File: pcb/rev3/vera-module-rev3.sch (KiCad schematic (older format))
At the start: 120 parts, among them J1 Bus, J2 Prog, J3 SD_Card, J4 Composite, J5 VGA, J6 Conn_01x04, J7 Conn_01x02, J8 RS232, J9 S-video, U1 ICE40UP5K-SG48ITR50, U10 MIC5504-3.3YM5, U11 THS7314D, U12 MAX3221CPWR, U2 74AHC00PW, U3 SN74CBTD3861PWR, U4 74AHC1G14GW,125, U5 74LVC4245APW, U6 WM8524CGEDT, U7 W25Q16JVSNIQ, U8 74AHC1G14GW,125, U9 AP3417CKTR-G1, X1 SG5032CAN_25.000000M-TJGA3

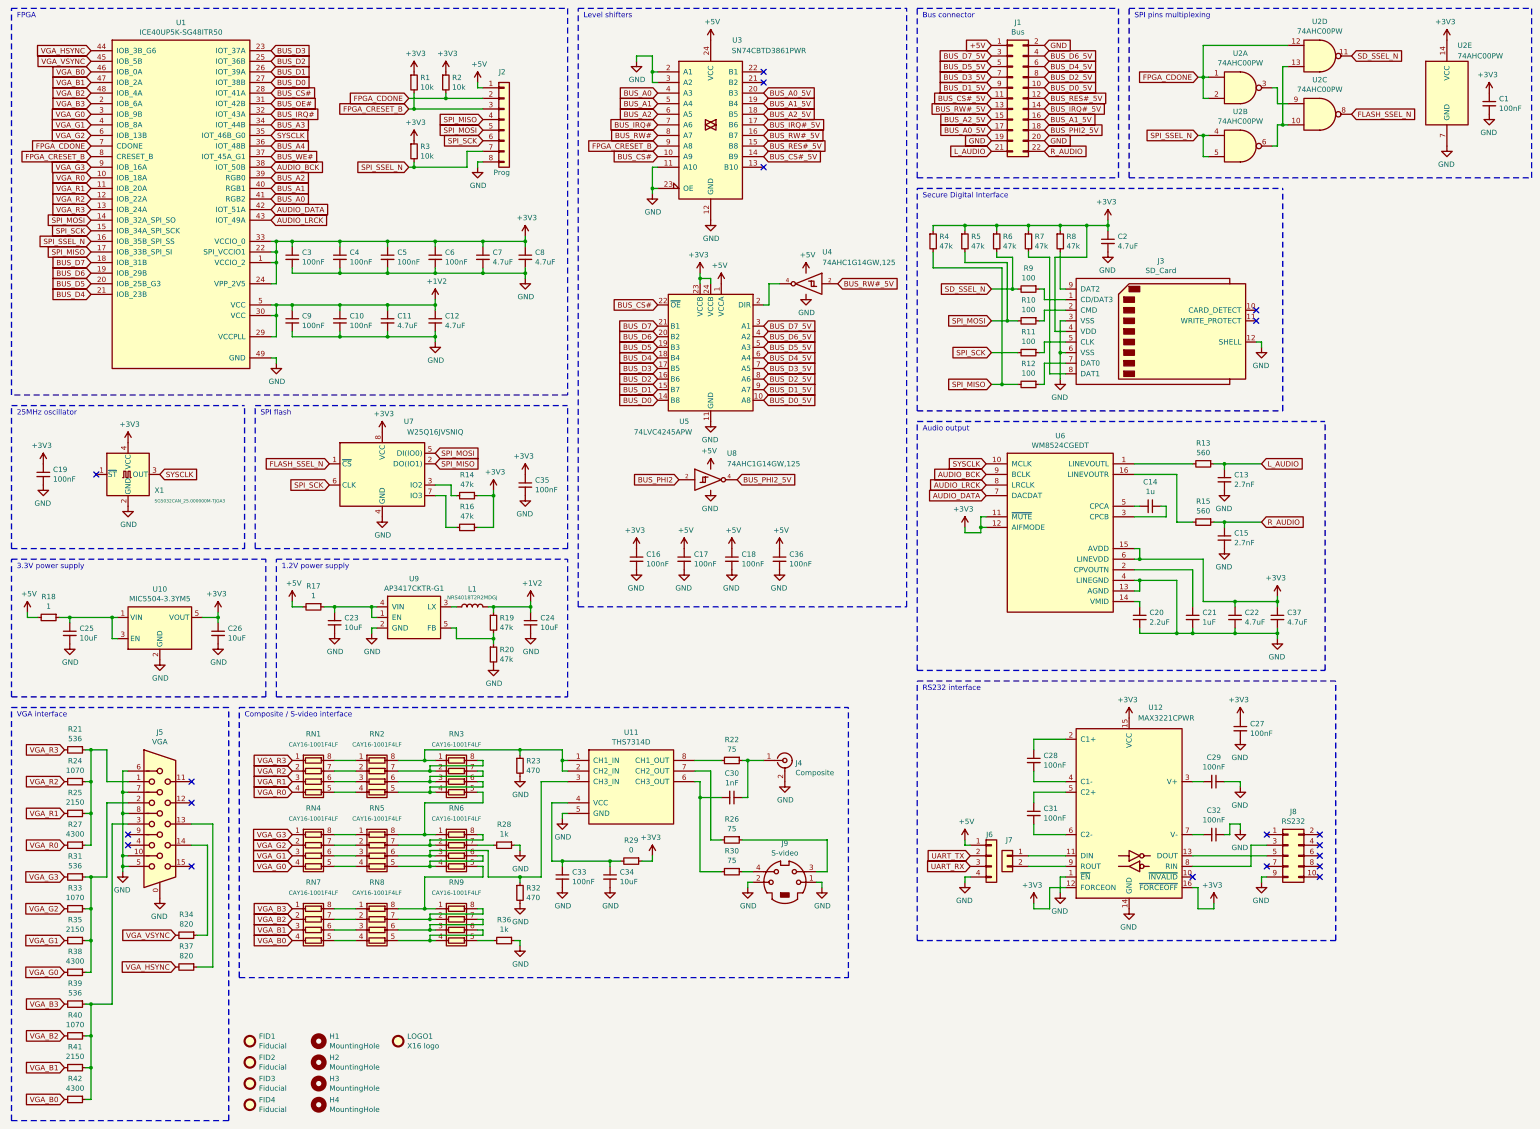
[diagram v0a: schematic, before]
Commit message: Worked on rev3 PCB.
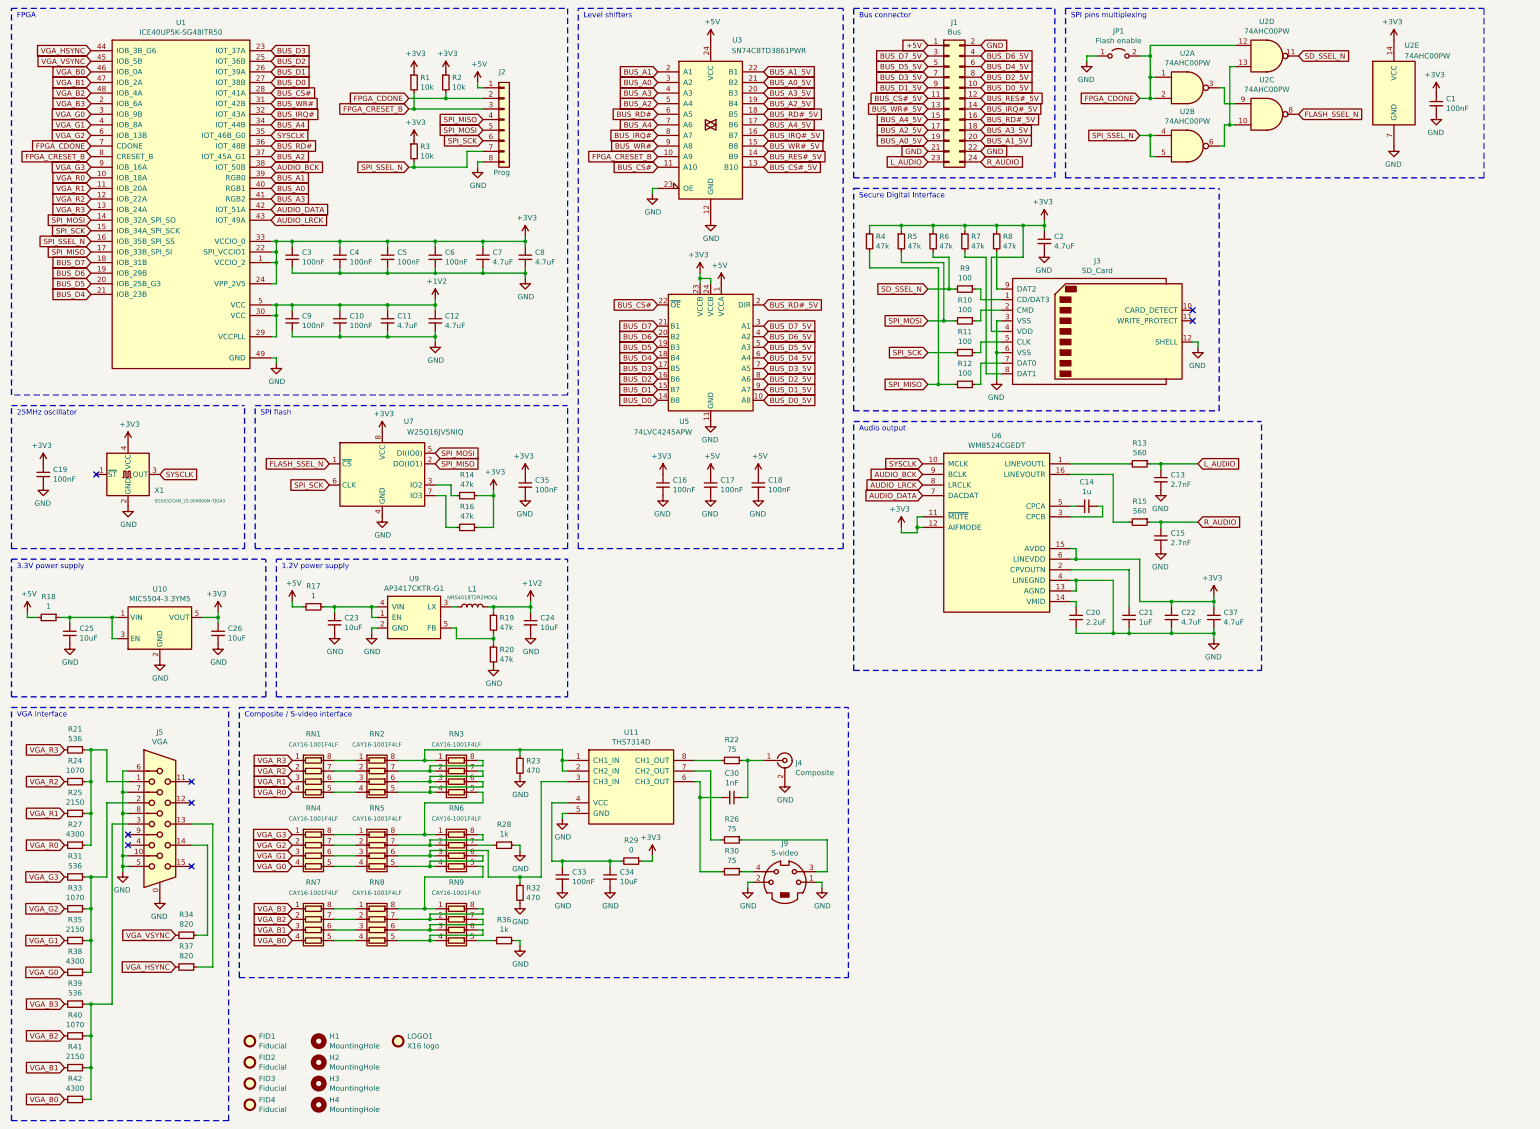
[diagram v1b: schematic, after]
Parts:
- removed C27, C28, C29, C31, C32, C36: 100nF, Capacitor_SMD:C_0603_1608Metric, symbol Device:C_Small
- removed J1: Bus, Connector_PinHeader_2.54mm:PinHeader_2x11_P2.54mm_Vertical, symbol Connector_Generic:Conn_02x11_Odd_Even
- removed J6: Conn_01x04, Connector_PinHeader_2.54mm:PinHeader_1x04_P2.54mm_Vertical, symbol Connector_Generic:Conn_01x04
- removed J7: Conn_01x02, Connector_PinHeader_2.54mm:PinHeader_1x02_P2.54mm_Vertical, symbol Connector_Generic:Conn_01x02
- removed J8: RS232, Connector_PinHeader_2.54mm:PinHeader_2x05_P2.54mm_Vertical, symbol Connector_Generic:Conn_02x05_Odd_Even
- removed U12: MAX3221CPWR, Package_SO:TSSOP-16_4.4x5mm_P0.65mm, symbol Interface_UART:MAX3221
- removed U4, U8: 74AHC1G14GW,125, Package_TO_SOT_SMD:SOT-353_SC-70-5, symbol 74xGxx:74AHCT1G14
- added J1: Bus, Connector_PinHeader_2.54mm:PinHeader_2x12_P2.54mm_Vertical, symbol Connector_Generic:Conn_02x12_Odd_Even
- added JP1: Flash enable, Connector_PinHeader_2.54mm:PinHeader_1x02_P2.54mm_Vertical, symbol Jumper:Jumper_2_Open
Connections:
- net BUS_RW# is gone; now on net BUS_IRQ#: U3.8 (A7)
- net BUS_RW#_5V is gone; now on net BUS_IRQ#_5V: U3.16 (B7)
- net BUS_WE# is gone; now on net BUS_A2: U1.37 (IOT_45A_G1)
- net +5V: now also J1.1 (Pin_1)
- net BUS_A0: now also U1.40 (RGB1), U3.3 (A2); no longer U1.41 (RGB2), U3.4 (A3)
- net BUS_A0_5V: now also U3.21 (B2), J1.19 (Pin_19); no longer U3.20 (B3)
- net BUS_A1: now also U1.39 (RGB0), U3.2 (A1); no longer U1.40 (RGB1), U3.5 (A4)
- net BUS_A1_5V: now also U3.22 (B1), J1.20 (Pin_20); no longer U3.19 (B4)
- net BUS_A2: now also U3.5 (A4); no longer U1.39 (RGB0), U3.6 (A5)
- net BUS_A2_5V: now also U3.19 (B4), J1.17 (Pin_17); no longer U3.18 (B5)
- net BUS_A3: now also U1.41 (RGB2), U3.4 (A3); no longer U1.34 (IOT_44B)
- net BUS_A4: now also U1.34 (IOT_44B), U3.7 (A6); no longer U1.36 (IOT_48B)
- net BUS_CS#: now also U3.11 (A10); no longer U3.10 (A9)
- net BUS_CS#_5V: now also U3.13 (B10), J1.11 (Pin_11); no longer U3.14 (B9)
- net BUS_D0_5V: now also J1.10 (Pin_10)
- net BUS_D1_5V: now also J1.9 (Pin_9)
- net BUS_D2_5V: now also J1.8 (Pin_8)
- net BUS_D3_5V: now also J1.7 (Pin_7)
- net BUS_D4_5V: now also J1.6 (Pin_6)
- net BUS_D5_5V: now also J1.5 (Pin_5)
- net BUS_D6_5V: now also J1.4 (Pin_4)
- net BUS_D7_5V: now also J1.3 (Pin_3)
- net BUS_IRQ#: no longer U3.7 (A6)
- net BUS_IRQ#_5V: now also J1.14 (Pin_14); no longer U3.17 (B6)
- net BUS_RES#_5V: now also U3.14 (B9), J1.12 (Pin_12); no longer U3.15 (B8)
- net FPGA_CDONE: now also JP1.2 (B)
- net FPGA_CRESET_B: now also U3.10 (A9); no longer U3.9 (A8)
- net GND: now also J1.2 (Pin_2), J1.21 (Pin_21), J1.22 (Pin_22), JP1.1 (A); no longer U3.11 (A10), U3.2 (A1), U3.3 (A2)
- net L_AUDIO: now also J1.23 (Pin_23)
- net R_AUDIO: now also J1.24 (Pin_24)
- net BUS_RD#_5V: now reaches U5.2 (DIR)
- net BUS_RD#_5V: now also U3.18 (B5), J1.16 (Pin_16)
- net BUS_OE# renamed BUS_WR#
- net BUS_WR#: now also U3.9 (A8)
- new net BUS_A3_5V: J1.18 (Pin_18), U3.20 (B3)
- new net BUS_A4_5V: J1.15 (Pin_15), U3.17 (B6)
- new net BUS_RD#: U1.36 (IOT_48B), U3.6 (A5)
- new net BUS_WR#_5V: J1.13 (Pin_13), U3.15 (B8)
- no-connect marks 19 -> 8
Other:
- note removed: "RS232 interface"
- moved on the sheet: C1, C13, C14, C15, C16, C17, C18, C2, C20, C21, C22, C37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

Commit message: Adding address decrement. Fixing port 1 address increment.
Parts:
- LOGO1: footprint vera-module:x16logo -> vera-module:x16plogo
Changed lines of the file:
@@
 Title "VERA module"
 Date "2020-02-14"
-Rev "2"
+Rev "3"
 Comp "(C) 2020 Frank van den Hoef"
 Comment1 ""
@@
 F 0 "LOGO1" H 4335 10396 50  0000 L CNN
 F 1 "X16 logo" H 4335 10305 50  0000 L CNN
-F 2 "vera-module:x16logo" H 4250 10350 50  0001 C CNN
+F 2 "vera-module:x16plogo" H 4250 10350 50  0001 C CNN
 F 3 "~" H 4250 10350 50  0001 C CNN
 	1    4250 10350
